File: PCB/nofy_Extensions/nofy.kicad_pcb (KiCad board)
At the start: 2 copper layers, 205.6 x 171.6 mm, 147 parts, among them J10 Conn_01x01-Connector_Generic, J11 Conn_01x01-Connector_Generic, J13 Conn_01x01-Connector_Generic, J14 Conn_01x01-Connector_Generic, J15 Conn_01x01-Connector_Generic, J16 Conn_01x01-Connector_Generic, J17 Conn_01x01-Connector_Generic, J18 Conn_01x01-Connector_Generic, J19 Conn_01x01-Connector_Generic, J21 Conn_01x01-Connector_Generic, J22 PIn1x4, J23 PIn1x4, J24 PIn1x4, J25 PIn1x4, J26 PIn1x4, J27 PIn1x4, J28 PIn1x4, J29 PIn1x4, J30 PIn1x4, J31 PIn1x4, J32 PIn1x4, J33 PIn1x4, J34 PIn1x4, J35 PIn1x4, J36 PIn1x4, J37 PIn1x4, J38 PIn1x4, J39 PIn1x4, J40 PIn1x4, J41 PIn1x4, SW1 RotaryEncoder, SW10 SW_PUSH, SW11 SW_PUSH, SW12 SW_PUSH, SW13 SW_PUSH, SW14 SW_PUSH, SW15 SW_PUSH, SW16 SW_PUSH, SW17 SW_PUSH, SW18 SW_PUSH, SW19 SW_PUSH, SW2 RotaryEncoder, SW20 SW_PUSH, SW21 SW_PUSH, SW22 SW_PUSH, SW23 SW_PUSH, SW24 SW_PUSH, SW25 SW_PUSH, SW26 SW_PUSH, SW27 SW_PUSH, SW28 SW_PUSH, SW29 SW_PUSH, SW3 SW_SPDT, SW30 SW_PUSH, SW31 SW_PUSH, SW32 SW_PUSH, SW33 SW_PUSH, SW34 SW_PUSH, SW35 SW_PUSH, SW36 SW_PUSH, SW37 SW_PUSH, SW38 SW_PUSH, SW39 SW_PUSH, SW4 SW_SPDT, SW40 SW_PUSH, SW41 SW_PUSH, SW42 SW_PUSH, SW43 SW_PUSH, SW44 SW_PUSH, SW45 SW_PUSH, SW46 SW_PUSH, SW47 SW_PUSH, SW48 SW_PUSH, SW49 SW_PUSH, SW5 SW_PUSH, SW50 SW_PUSH, SW51 SW_PUSH, SW52 SW_PUSH, SW53 SW_PUSH, SW54 SW_PUSH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

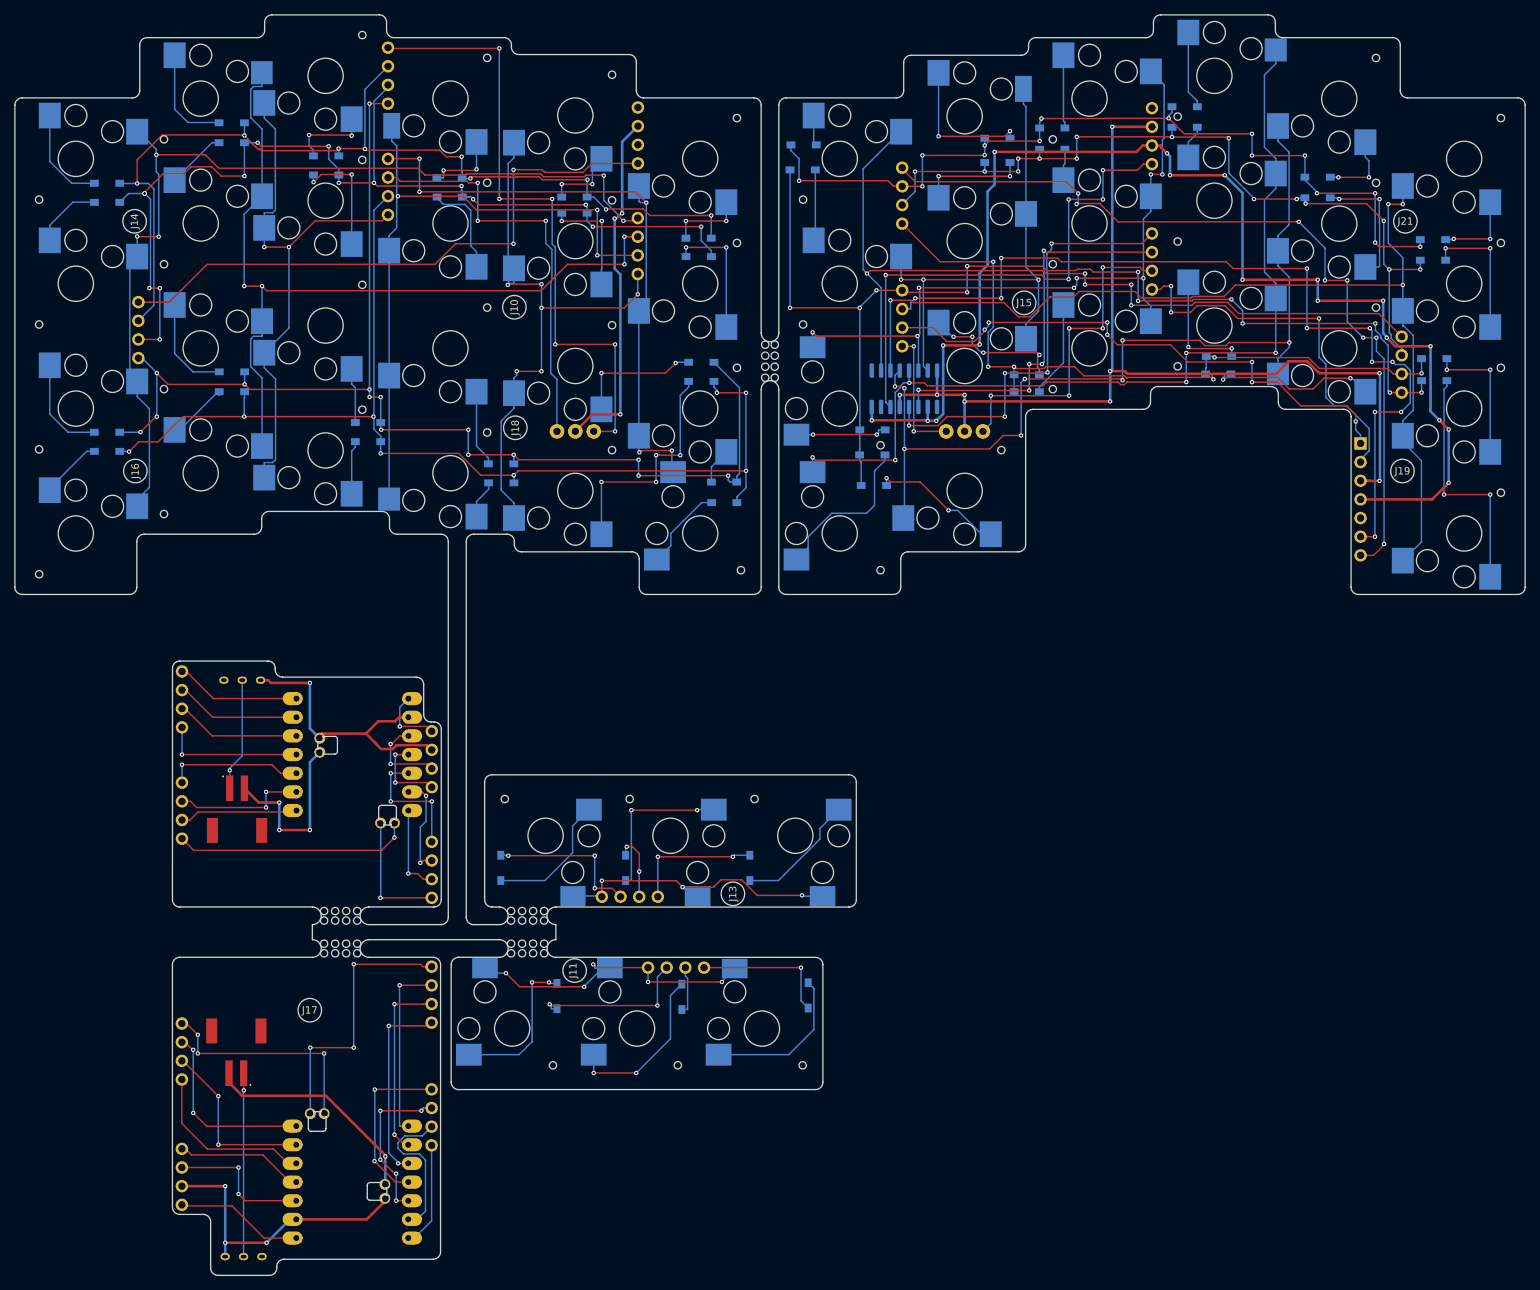
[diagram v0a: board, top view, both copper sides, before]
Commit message: Update : PCB
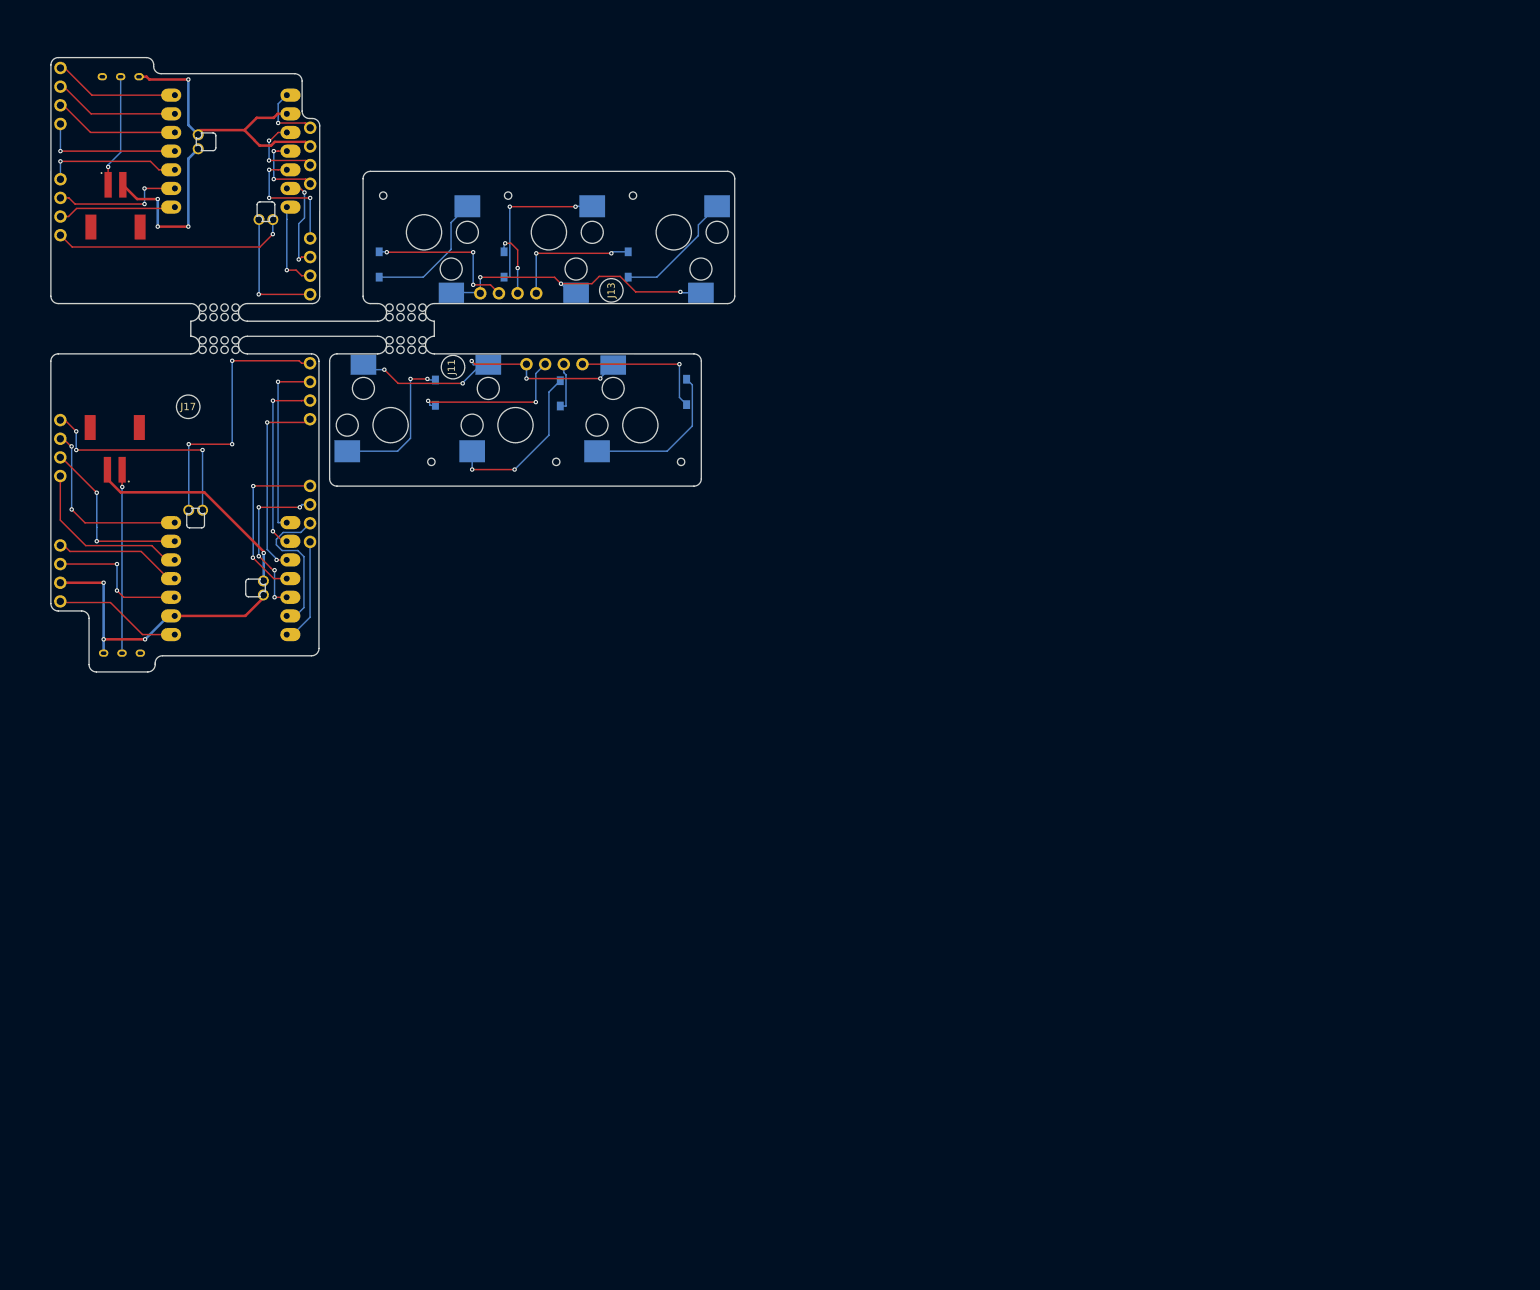
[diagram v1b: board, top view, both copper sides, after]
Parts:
- removed D1, D10, D11, D12, D13, D14, D15, D16, D17, D18, D19, D2, D20, D21, D28, D29, D3, D30, D31, D32, D33, D34, D35, D36, D37, D38, D39, D4, D40, D41, D42, D43, D44, D45, D46, D47, D48, D49, D5, D50, D51, D6, D7, D8, D9: D, _kicad_footprints:Diode_SMD
- removed J10, J14, J15, J16, J18, J19, J21: Conn_01x01-Connector_Generic, MountingHole:MountingHole_3.2mm_M3
- removed J2: ~, _kicad_footprints:pmw3610_connector
- removed J22, J25, J27, J29, J30, J32, J36, J37, J38, J39: PIn1x4, nofy:Pin1x4
- removed REF**1: StampHole, nofy:StampHole
- removed SW1, SW2: RotaryEncoder, nofy:RotaryEncoder_EC12E
- removed SW10, SW11, SW12, SW13, SW14, SW15, SW16, SW17, SW18, SW19, SW20, SW21, SW22, SW23, SW24, SW25, SW32, SW33, SW34, SW35, SW36, SW37, SW38, SW39, SW40, SW41, SW42, SW43, SW44, SW45, SW46, SW47, SW48, SW49, SW5, SW50, SW51, SW52, SW53, SW54, SW55, SW6, SW7, SW8, SW9: SW_PUSH, nofy:Choc_v2_Hotswap_1u_17mm
- removed U3: 74HC595, Package_SO:SOIC-16_3.9x9.9mm_P1.27mm
- moved B1 83.8 mm to (30.2, 41.8)
- moved BT1 83.8 mm to (30.1, 80.6)
- moved D22 83.8 mm to (73.8, 72.9)
- moved D23 83.8 mm to (90.8, 73.0)
- moved D24 83.8 mm to (108.0, 72.8)
- moved D25 83.8 mm to (66.1, 49.9)
- moved D26 83.8 mm to (83.1, 49.9)
- moved D27 83.8 mm to (100.0, 49.9)
- moved J13 83.8 mm to (97.7, 56.2)
- moved J26 83.8 mm to (55.4, 32.8)
- moved J28 83.8 mm to (55.4, 47.8)
- moved J33 83.8 mm to (21.4, 39.8)
- moved J34 83.8 mm to (24.0, 99.8)
- moved J35 83.8 mm to (24.0, 82.8)
- moved J40 83.8 mm to (58.0, 91.7)
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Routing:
- net 3.3V: track 171.7 -> 0.00 mm, vias 18 -> 0
- net Row7: track 169.4 -> 0.00 mm, vias 15 -> 0
- net Row3: track 150.5 -> 0.00 mm, vias 12 -> 0
- net Row8: track 149.6 -> 0.00 mm, vias 8 -> 0
- net Col4: track 139.9 -> 0.00 mm, vias 4 -> 0
- net Row6: track 138.5 -> 0.00 mm, vias 15 -> 0
- net GND_R: track 137.0 -> 0.00 mm, vias 9 -> 0
- net Row5: track 133.3 -> 0.00 mm, vias 9 -> 0
- net Col7: track 129.4 -> 0.00 mm, vias 5 -> 0
- net Col2: track 125.2 -> 0.00 mm, vias 6 -> 0
- net Col3: track 124.4 -> 0.00 mm, vias 8 -> 0
- net SDIO: track 118.0 -> 0.00 mm, vias 11 -> 0
- net Row0: track 117.7 -> 0.00 mm, vias 15 -> 0
- net Col5: track 115.3 -> 0.00 mm, vias 5 -> 0
- net Col8: track 114.8 -> 0.00 mm, vias 4 -> 0
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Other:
- board size 205.6 x 171.6 mm -> 93.1 x 83.6 mm
- board text removed: "nofy V2"

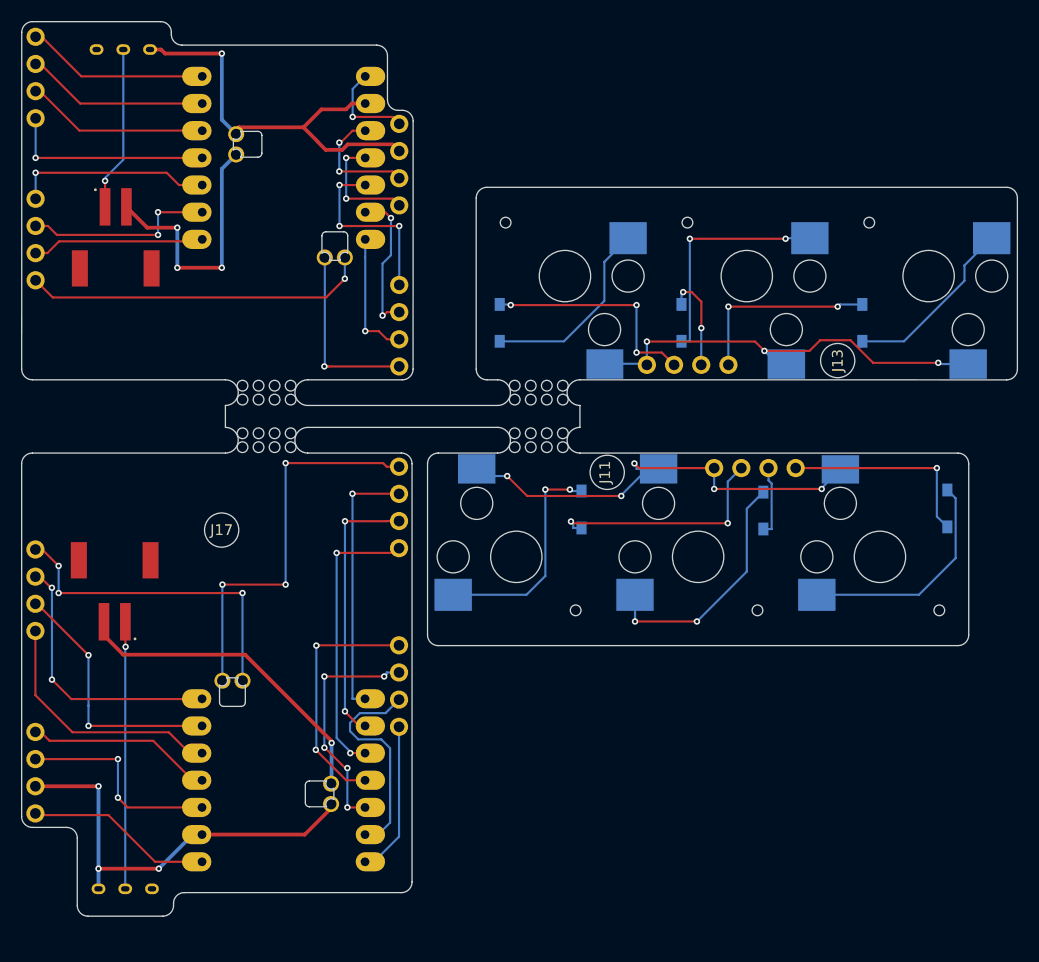
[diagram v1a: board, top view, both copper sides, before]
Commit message: Update : PCB
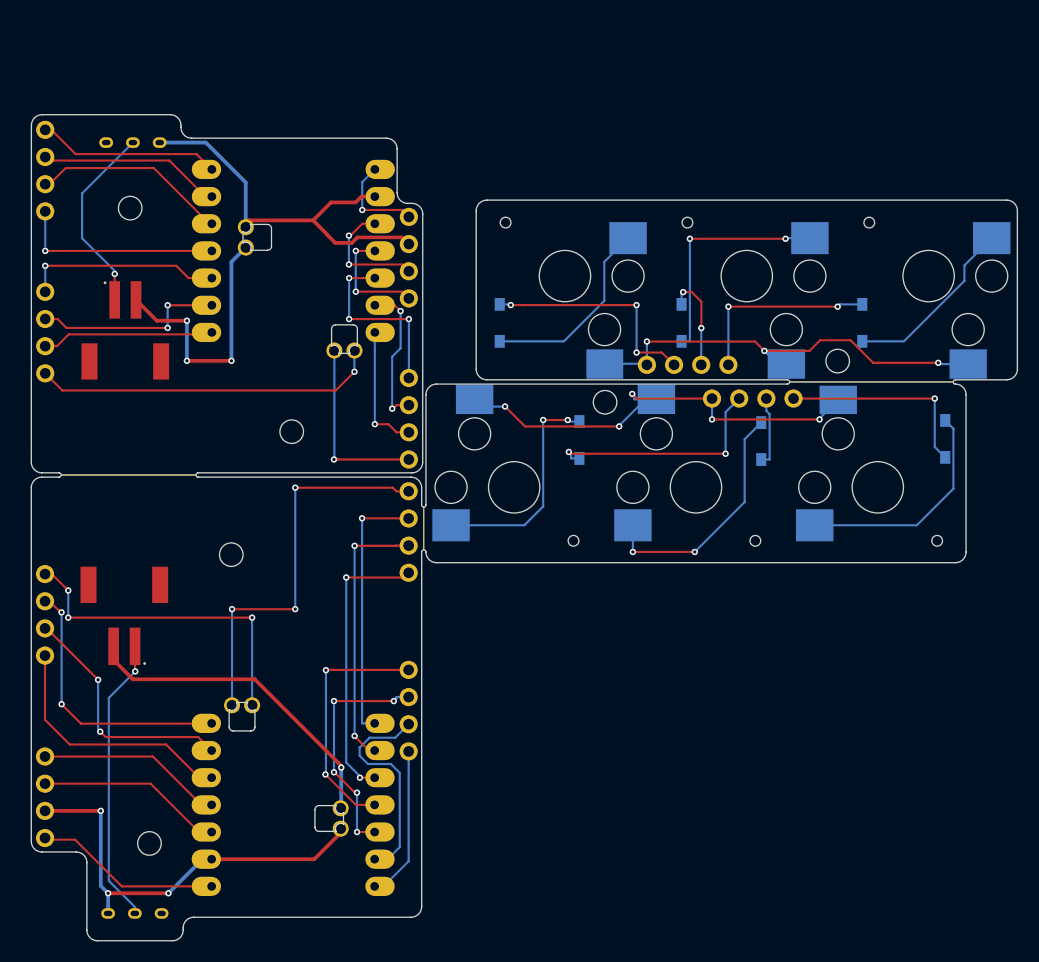
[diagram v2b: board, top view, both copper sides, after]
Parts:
- removed J11, J13, J17: Conn_01x01-Connector_Generic, MountingHole:MountingHole_3.2mm_M3
- removed REF**4, REF**5: StampHole, nofy:StampHole
- added REF**1: MountingHole_2.2mm_M2, nofy:MountingHole_2.2mm_M2, F.Cu at (31.6, 42.0)
- added REF**12: MountingHole_2.2mm_M2, nofy:MountingHole_2.2mm_M2, F.Cu at (76.0, 60.1)
- added REF**13: MountingHole_2.2mm_M2, nofy:MountingHole_2.2mm_M2, F.Cu at (41.0, 74.3)
- added REF**14: MountingHole_2.2mm_M2, nofy:MountingHole_2.2mm_M2, F.Cu at (33.4, 101.3)
- REF**2, REF**3: value StampHole -> MountingHole_2.2mm_M2; footprint nofy:StampHole -> nofy:MountingHole_2.2mm_M2
- moved REF**3 28.1 mm to (97.7, 56.2), turned to 0 degrees
- moved J26 8.75 mm to (56.3, 41.5)
- moved J28 8.75 mm to (56.3, 56.5)
- moved B1 8.75 mm to (31.1, 50.5)
- moved J33 8.75 mm to (22.3, 48.5)
- moved SW3 8.75 mm to (31.8, 33.1)
- moved J31 8.75 mm to (22.3, 33.3)
- moved U2 8.75 mm to (46.8, 35.5)
- moved D22 6.50 mm to (73.5, 66.4)
- moved D23 6.50 mm to (90.5, 66.5)
- moved D24 6.50 mm to (107.8, 66.3)
- moved J23 6.50 mm to (84.7, 61.1)
- moved SW26 6.50 mm to (67.5, 68.1)
- moved SW27 6.50 mm to (84.5, 68.1)
- moved SW28 6.50 mm to (101.5, 68.1)
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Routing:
- net Net-(B1--): track 15.4 -> 17.9 mm
- net Net-(J34-Pin_3): track 19.6 -> 17.5 mm, vias 2 -> 0
- net Net-(BT1--): track 25.0 -> 27.0 mm
- net Net-(J31-Pin_3): track 17.1 -> 18.4 mm
- net GND_L_b: track 38.8 -> 37.6 mm, vias 1 -> 0
- net Net-(J35-Pin_2): track 24.2 -> 23.1 mm
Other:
- board size 93.1 x 83.6 mm -> 92.2 x 77.2 mm
- board text added: "L"
- board text added: "R"
